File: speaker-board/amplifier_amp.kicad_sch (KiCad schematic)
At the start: 23 parts, among them J2 OUPUT+, J3 OUTPUT-, J4 V+, J5 GND, J6 V-, U1 LM3886

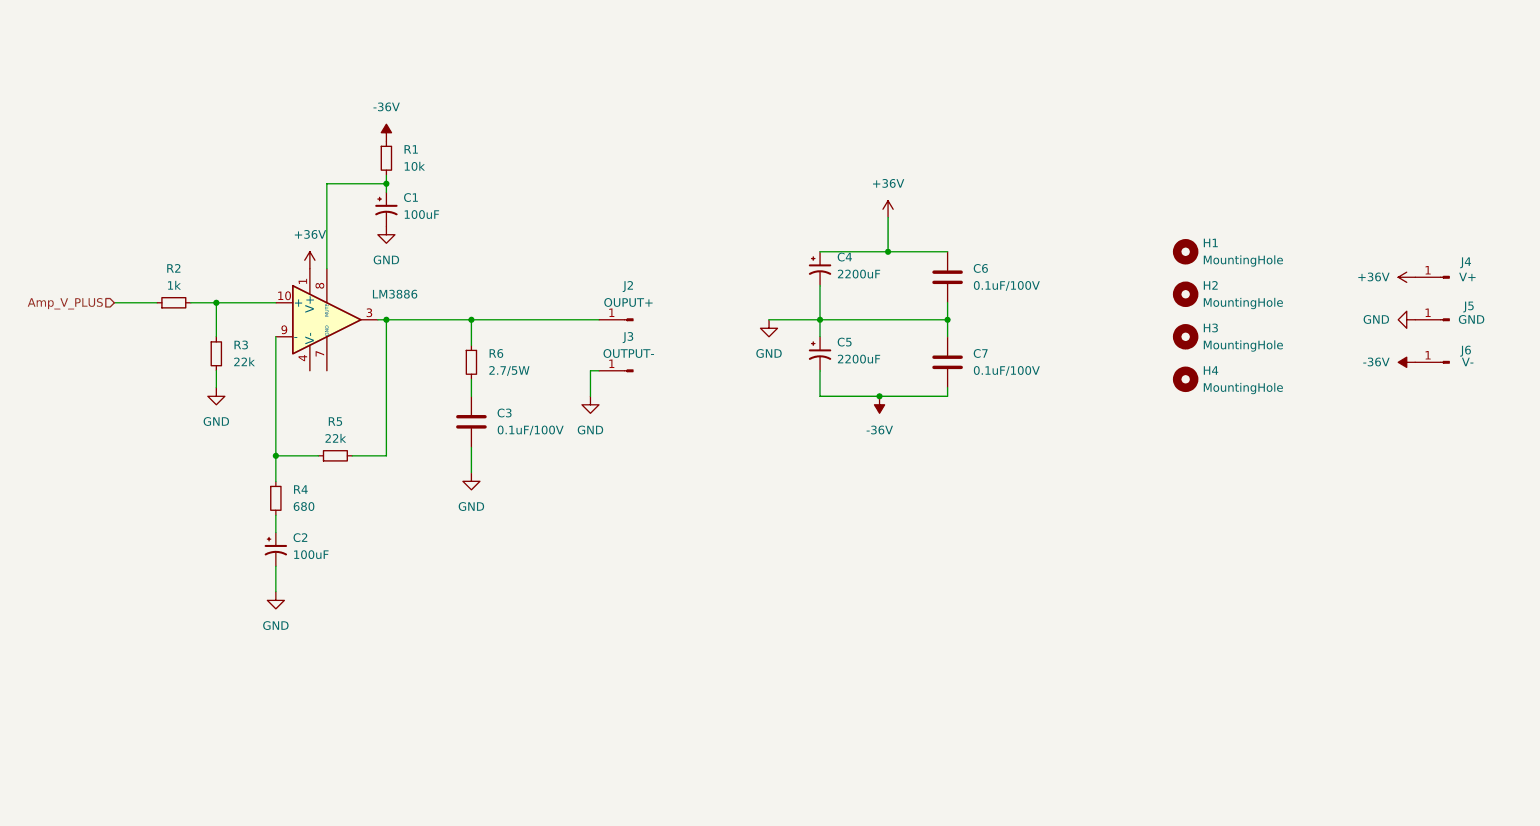
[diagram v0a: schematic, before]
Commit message: updated
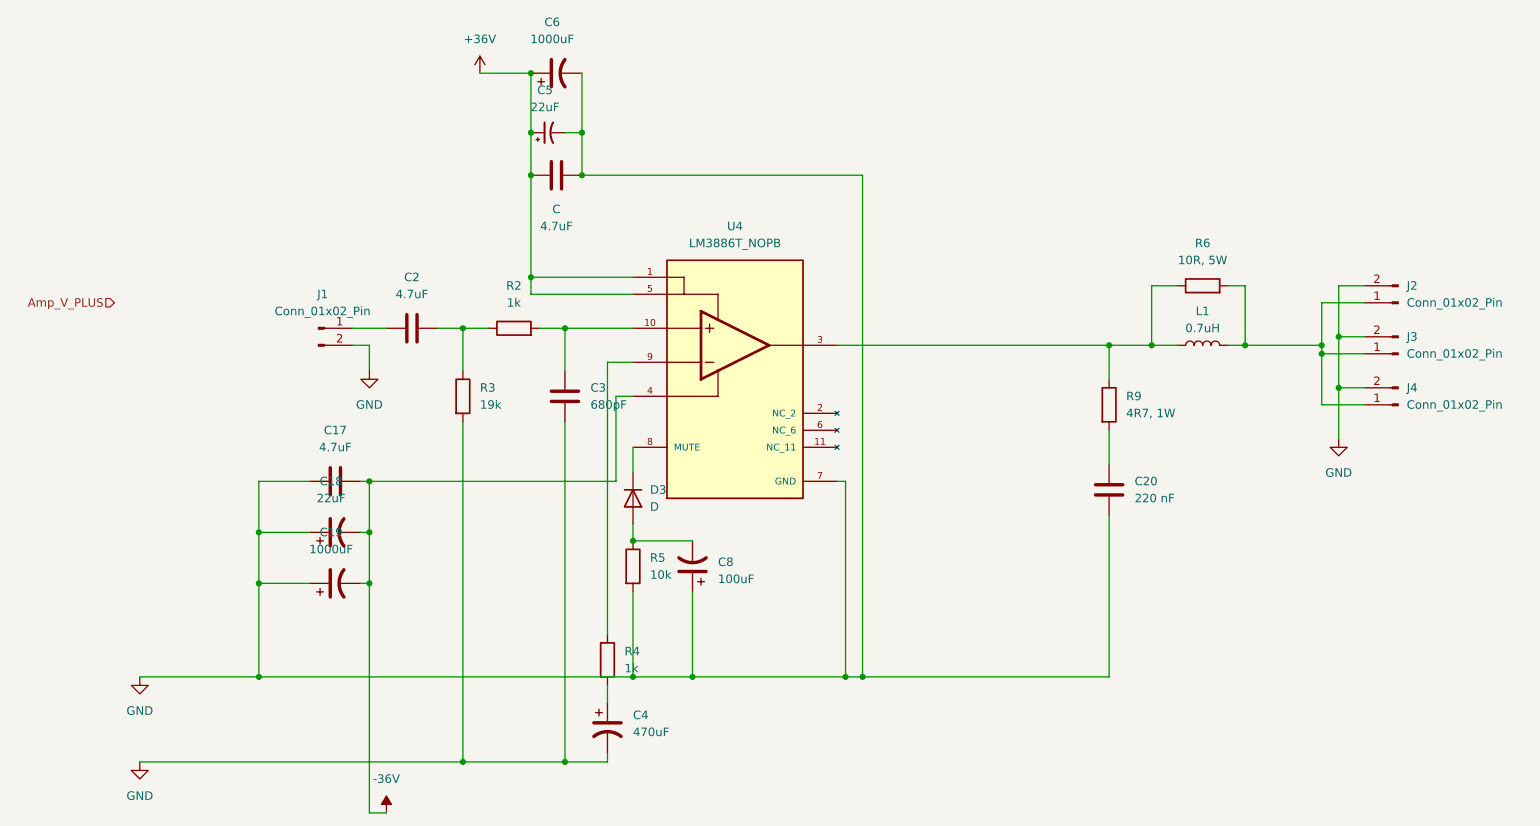
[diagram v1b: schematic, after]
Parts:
- removed C1, C2: 100uF, symbol Device:C_Polarized_Small_US
- removed C4: 2200uF, symbol Device:C_Polarized_Small_US
- removed C6, C7: 0.1uF/100V, symbol Device:C
- removed H1, H2, H3, H4: MountingHole, symbol Mechanical:MountingHole
- removed J2: OUPUT+, symbol Connector:Conn_01x01_Pin
- removed J3: OUTPUT-, symbol Connector:Conn_01x01_Pin
- removed J4: V+, symbol Connector:Conn_01x01_Pin
- removed J5: GND, symbol Connector:Conn_01x01_Pin
- removed J6: V-, symbol Connector:Conn_01x01_Pin
- removed R1: 10k, symbol Device:R_Small
- removed R2: 1k, symbol Device:R_Small
- removed R3, R5: 22k, symbol Device:R_Small
- removed R4: 680, symbol Device:R_Small
- removed R6: 2.7/5W, symbol Device:R_Small
- removed U1: LM3886, Package_TO_SOT_THT:TO-220-11_P3.4x5.08mm_StaggerOdd_Lead4.85mm_Vertical, symbol Amplifier_Audio:LM3886
- added 4.7uF: C, symbol Device:C
- added C17, C2: 4.7uF, symbol Device:C
- added C18: 22uF, symbol Device:C_Polarized_US
- added C19, C6: 1000uF, symbol Device:C_Polarized_US
- added C20: 220 nF, symbol Device:C
- added C4: 470uF, symbol Device:C_Polarized_US
- added C8: 100uF, symbol Device:C_Polarized_US
- added D3: D, symbol Device:D
- added J1, J2, J3, J4: Conn_01x02_Pin, symbol Connector:Conn_01x02_Pin
- added L1: 0.7uH, symbol Device:L
- added R2, R4: 1k, symbol Device:R
- added R3: 19k, symbol Device:R
- added R5: 10k, symbol Device:R
- added R6: 10R, 5W, symbol Device:R
- added R9: 4R7, 1W, symbol Device:R
- added U4: LM3886T_NOPB, LM3886T_NOPB:TO170P2027X462X2082-11, symbol LM3886T_NOPB:LM3886T_NOPB
- C3: value 0.1uF/100V -> 680pF
- C5: value 2200uF -> 22uF
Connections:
- net +36V: now also C5.1, 4.7uF.1, C6.1, U4.1, U4.5
- net -36V: now also C17.2, C18.2, C19.2, U4.4; no longer C5.2
- net GND: now also C5.2, 4.7uF.2, C17.1, C18.1, C19.1, C20.2, C4.2, C6.2, C8.1, J1.2 (Pin_2), J2.2 (Pin_2), J3.2 (Pin_2), J4.2 (Pin_2), R3.2, R5.2, U4.7 (GND); no longer C5.1
- net at C3.1: now also R2.2, U4.10
- new net: C8.2, D3.2 (A), R5.1
- new net: J2.1 (Pin_1), J3.1 (Pin_1), J4.1 (Pin_1), L1.2, R6.2
- new net: L1.1, R6.1, R9.1, U4.3
- new net: C4.1, R4.2
- new net: R4.1, U4.9
- new net: C2.1, R2.1, R3.1
- new net: C2.2, J1.1 (Pin_1)
- new net: C20.1, R9.2
- new net: D3.1 (K), U4.8 (MUTE)
